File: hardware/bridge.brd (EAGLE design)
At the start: 37.8 x 90.2 mm, 21 parts, among them IC1 MC34063AP, IC2 MAX3232CPE, J1 RJ11, J2 RJ9PTH, M1 ESP01

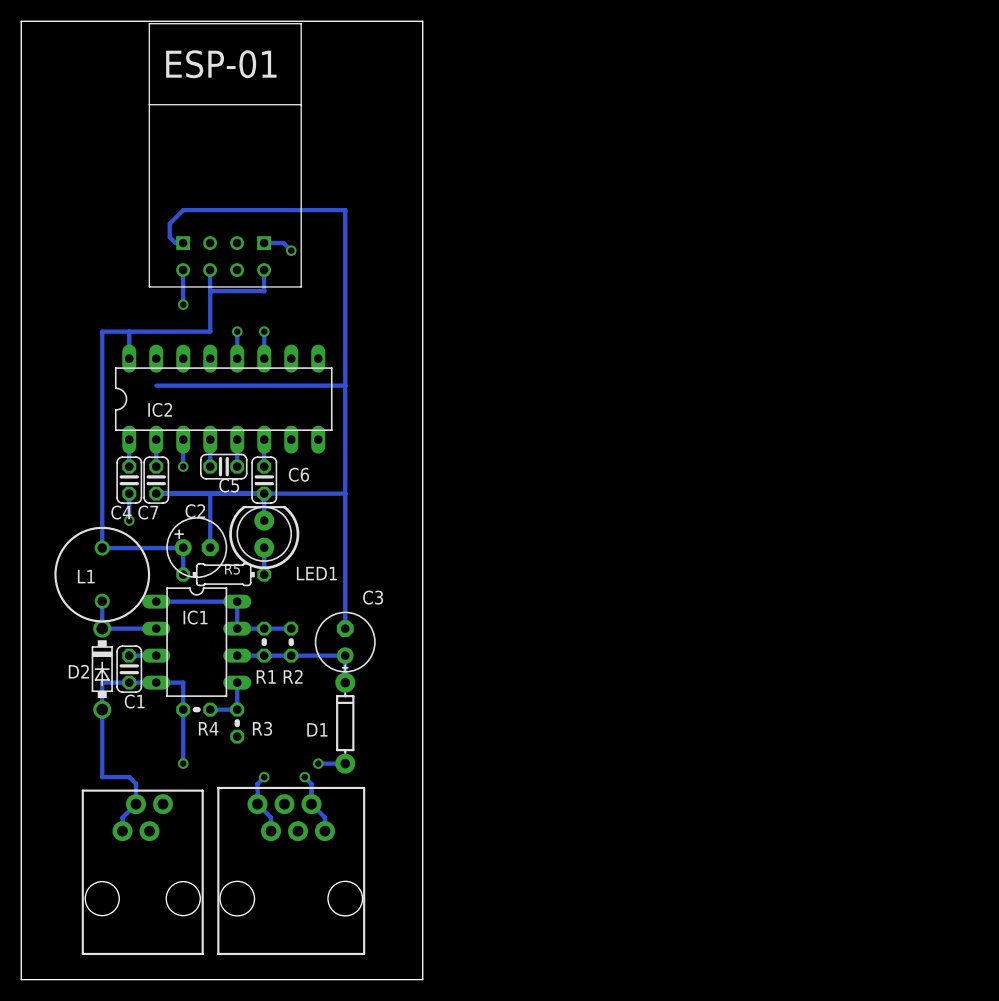
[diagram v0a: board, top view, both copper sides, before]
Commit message: Small board changes
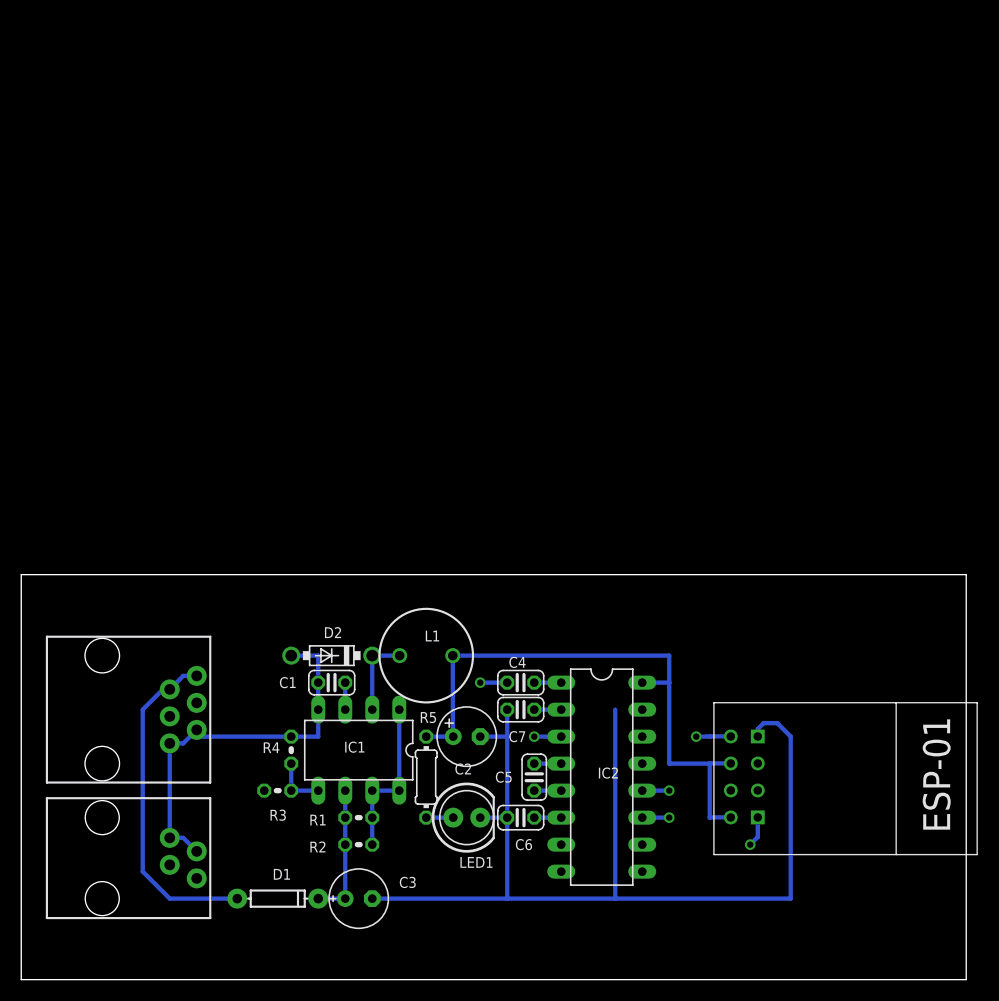
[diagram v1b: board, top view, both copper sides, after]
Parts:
- moved M1 79.0 mm to (74.9, 19.1), turned to 270 degrees
- moved IC2 50.3 mm to (54.6, 19.1), turned to 270 degrees
- moved C4 41.5 mm to (47.0, 27.9), turned to 180 degrees
- moved C5 41.3 mm to (48.3, 19.1), turned to 270 degrees
- moved C7 40.5 mm to (47.0, 25.4), turned to 180 degrees
- moved C6 39.9 mm to (47.0, 15.2), turned to 180 degrees
- moved LED1 32.8 mm to (41.9, 15.2), turned to 0 degrees
- moved L1 31.4 mm to (38.1, 30.5), turned to 0 degrees
- moved C2 31.0 mm to (41.9, 22.9)
- moved R5 26.9 mm to (38.1, 19.1), turned to 270 degrees
- moved J1 25.1 mm to (7.62, 25.4), turned to 270 degrees
- moved C3 24.2 mm to (31.8, 7.62), turned to 0 degrees
- moved D2 21.6 mm to (29.2, 30.5), turned to 180 degrees
- moved R2 20.1 mm to (31.8, 12.7), turned to 180 degrees
- moved C1 19.1 mm to (29.2, 27.9), turned to 180 degrees
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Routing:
- net VBATT: track 8.41 -> 31.6 mm, vias 2 -> 0
- net GND: track 150.9 -> 136.7 mm, vias 2 -> 0
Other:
- board size 37.8 x 90.2 mm -> 88.9 x 38.1 mm
